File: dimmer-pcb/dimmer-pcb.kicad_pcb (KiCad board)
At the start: 2 copper layers, 13 parts, among them J3 Conn_01x04, Q1 BT136, U1 PC817, U3 MOC3021M

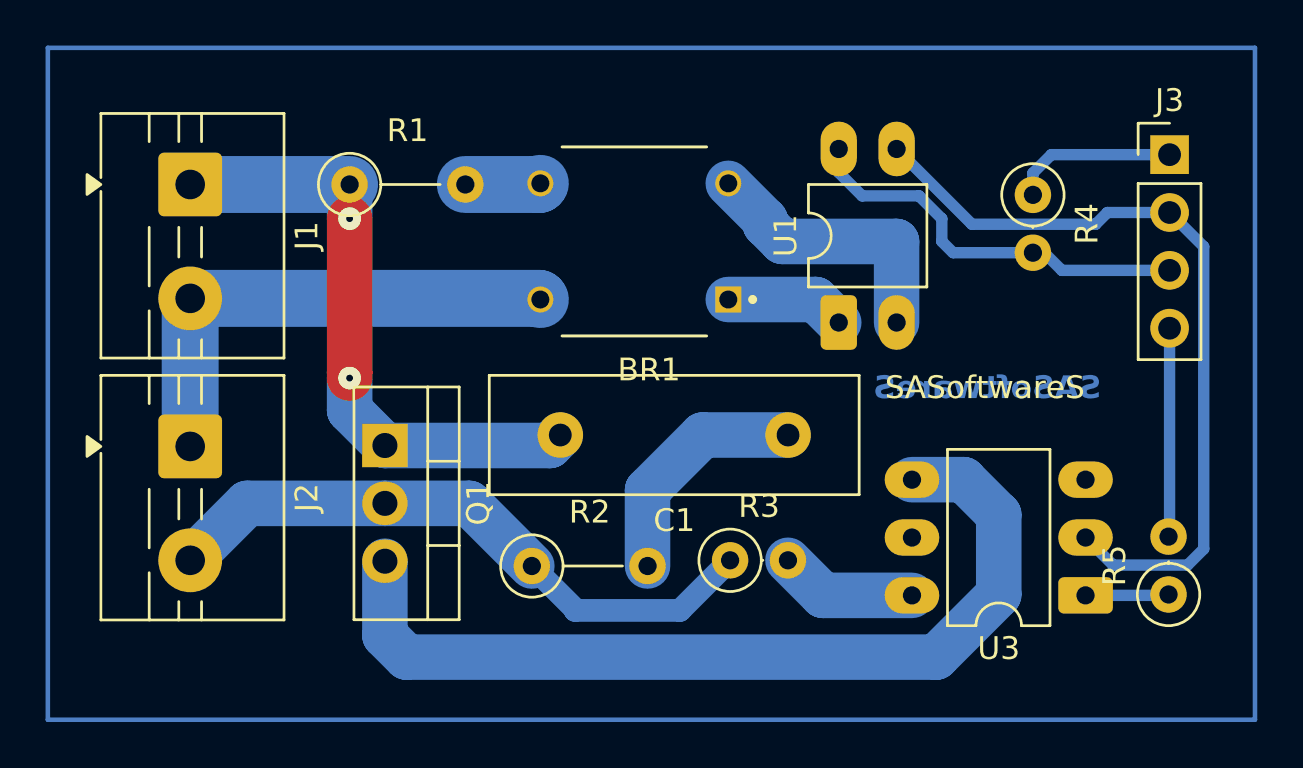
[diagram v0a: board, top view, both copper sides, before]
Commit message: Add files via upload
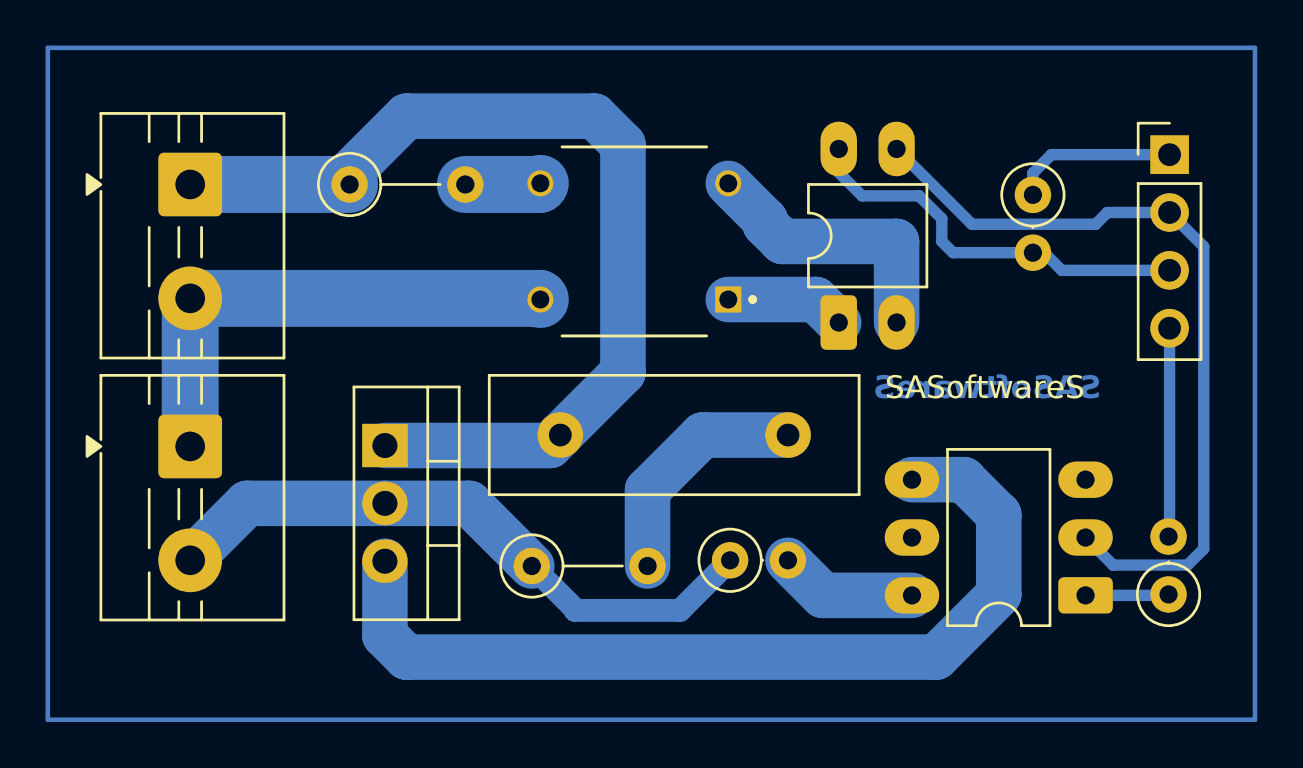
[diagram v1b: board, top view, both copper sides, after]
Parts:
- U3: value MOC3021M -> MOC3021
- renumbered BR1 to DB107
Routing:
- net Net-(J1-Pin_1): track 27.0 -> 42.8 mm, vias 2 -> 0
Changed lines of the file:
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@@
 			(at 2.25 -5.12 90)
 			(layer "F.SilkS")
+			(hide yes)
 			(effects
 				(font
@@
 			(at 0 -2.38 0)
 			(layer "F.SilkS")
+			(hide yes)
 			(effects
 				(font
@@
 			(at 2.54 -4.1 90)
 			(layer "F.SilkS")
+			(hide yes)
 			(effects
 				(font
@@
 			(at 2.54 -2.37 0)
 			(layer "F.SilkS")
+			(hide yes)
 			(effects
 				(font
@@
 			(at 1.27 -2.37 90)
 			(layer "F.SilkS")
+			(hide yes)
 			(effects
 				(font
@@
 			(at 1.27 -2.37 0)
 			(layer "F.SilkS")
+			(hide yes)
 			(effects
 				(font
@@
 			(at 3.81 -2.33 0)
 			(layer "F.SilkS")
+			(hide yes)
 			(effects
 				(font
@@
 			)
 		)
-		(property "Value" "MOC3021M"
+		(property "Value" "MOC3021"
 			(at 3.81 7.41 0)
 			(layer "F.Fab")
@@
 			(at 3.81 -2.33 90)
 			(layer "F.SilkS")
+			(hide yes)
 			(effects
 				(font
@@
 			(at 5 -3.75 0)
 			(layer "F.SilkS")
+			(hide yes)
 			(effects
 				(font
@@
 		)
 		(property "Value" "104J"
-			(at 5 3.75 0)
+			(at 4.75 1.5 0)
 			(layer "F.Fab")
 			(effects
@@
 			(at 2.25 -5.12 90)
 			(layer "F.SilkS")
+			(hide yes)
 			(effects
 				(font
@@
 		(layer "F.Cu")
 		(at 115 115 180)
-		(property "Reference" "BR1"
+		(property "Reference" "DB107"
 			(at -0.645 -5.635 0)
 			(layer "F.SilkS")
+			(hide yes)
 			(effects
 				(font
@@
 		)
 		(property "Value" "DB107"
-			(at 10.785 5.635 0)
+			(at -0.25 -2 0)
 			(layer "F.Fab")
 			(effects
@@
 			(at 1.27 -2.37 90)
 			(layer "F.SilkS")
+			(hide yes)
 			(effects
 				(font
@@
 			(at 2.54 -2.37 0)
 			(layer "F.SilkS")
+			(hide yes)
 			(effects
 				(font
@@
 	)
 	(segment
-		(start 102.5 120.75)
-		(end 102.5 121)
+		(start 114.5 120.75)
+		(end 111.75 123.5)
 		(width 2)
-		(layer "F.Cu")
+		(layer "B.Cu")
 		(net "Net-(J1-Pin_1)")
 	)
 	(segment
-		(start 102.5 114)
-		(end 102.5 120.75)
+		(start 102.5 112)
+		(end 105 109.5)
 		(width 2)
-		(layer "F.Cu")
-		(net "Net-(J1-Pin_1)")
-	)
-	(via
-		(at 102.5 121)
-		(size 1)
-		(drill 0.3)
-		(layers "F.Cu" "B.Cu")
+		(layer "B.Cu")
 		(net "Net-(J1-Pin_1)")
 	)
-	(via
-		(at 102.5 114)
-		(size 1)
-		(drill 0.3)
-		(layers "F.Cu" "B.Cu")
+	(segment
+		(start 111.29 123.96)
+		(end 111.75 123.5)
+		(width 2)
+		(layer "B.Cu")
 		(net "Net-(J1-Pin_1)")
 	)
 	(segment
-		(start 102.5 122.41)
-		(end 104.05 123.96)
+		(start 113.25 109.5)
+		(end 114.5 110.75)
 		(width 2)
 		(layer "B.Cu")
@@
 	)
 	(segment
-		(start 111.29 123.96)
-		(end 111.75 123.5)
+		(start 104.05 123.96)
+		(end 111.29 123.96)
 		(width 2)
 		(layer "B.Cu")
@@
 	)
 	(segment
-		(start 102.5 112.5)
-		(end 102.5 114)
+		(start 114.5 110.75)
+		(end 114.5 120.75)
 		(width 2)
 		(layer "B.Cu")
@@
 	)
 	(segment
-		(start 104.05 123.96)
-		(end 111.29 123.96)
+		(start 102.5 112.5)
+		(end 102.5 112)
 		(width 2)
 		(layer "B.Cu")
@@
 	)
 	(segment
-		(start 102.5 121)
-		(end 102.5 122.41)
+		(start 105 109.5)
+		(end 113.25 109.5)
 		(width 2)
 		(layer "B.Cu")
